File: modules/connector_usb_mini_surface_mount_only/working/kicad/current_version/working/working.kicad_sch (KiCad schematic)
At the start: 1 part, among them J1 scumnsmo

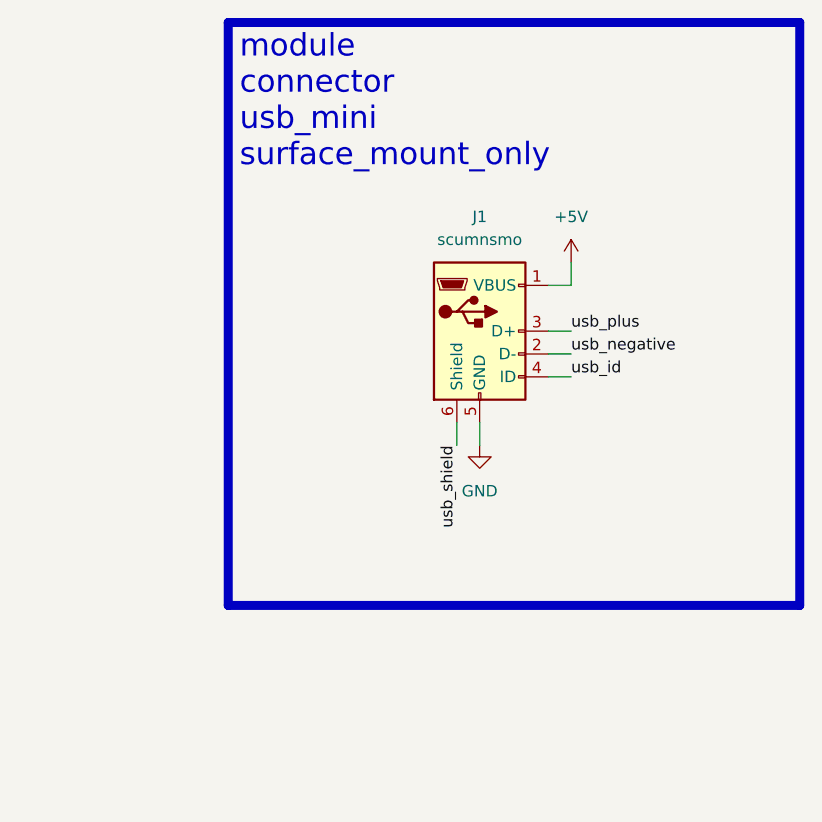
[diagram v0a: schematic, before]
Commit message: a few module workings
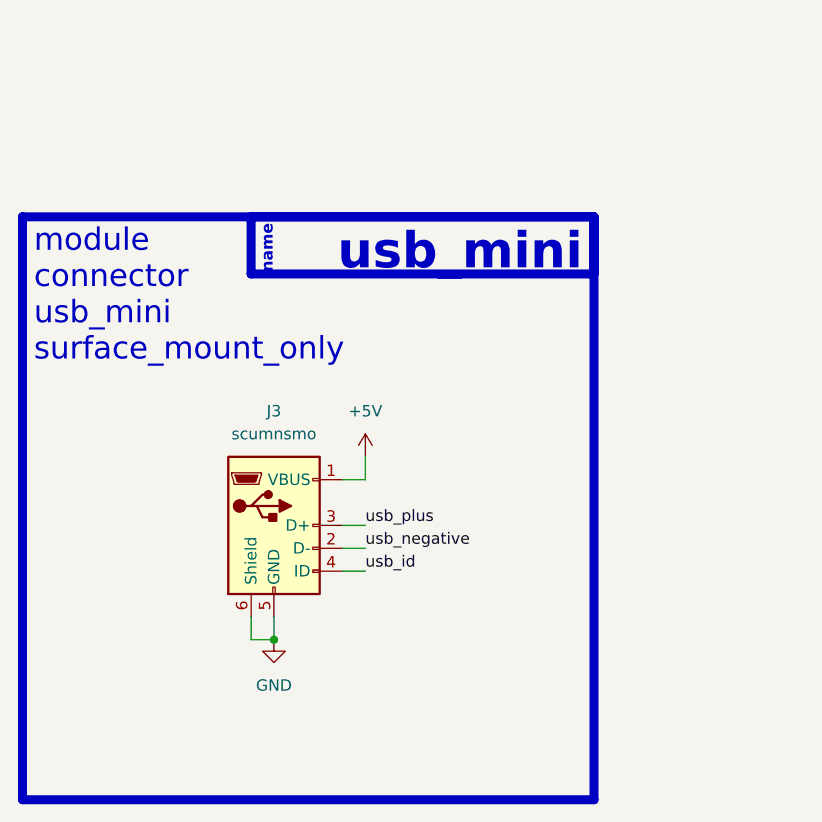
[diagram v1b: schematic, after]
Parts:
- removed J1: scumnsmo, scumnsmo_electronic_socket_usb_mini_surface_mount_only, symbol oomlout_oomp_part_symbols:scumnsmo_electronic_socket_usb_mini_surface_mount_only
- added J3: scumnsmo, oomlout_oomp_part_kicad_footprints:scumnsmo_electronic_socket_usb_mini_surface_mount_only, symbol oomlout_oomp_part_symbols:scumnsmo_electronic_socket_usb_mini_surface_mount_only
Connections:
- net +5V: now also J3.1 (VBUS)
- net GND: now also J3.5 (GND), J3.6 (Shield)
- net usb_id: now also J3.4 (ID)
- net usb_negative: now also J3.2 (D-)
- net usb_plus: now also J3.3 (D+)
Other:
- note added: "name"
- note added: "usb_mini"
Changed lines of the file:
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@@
 (kicad_sch (version 20230121) (generator eeschema)
   (paper "A4")
-  (wire (pts (xy 175.26 69.85) (xy 172.72 69.85))
+  (junction (at 142.24 109.22) (diameter 0) (color 0 0 0 0)
+  )
+  (wire (pts (xy 149.86 96.52) (xy 152.4 96.52))
     (stroke (width 0) (type default))
   )
-  (wire (pts (xy 165.1 85.09) (xy 165.1 87.63))
+  (wire (pts (xy 142.24 106.68) (xy 142.24 109.22))
     (stroke (width 0) (type default))
   )
-  (wire (pts (xy 162.56 85.09) (xy 162.56 87.63))
+  (wire (pts (xy 152.4 91.44) (xy 149.86 91.44))
     (stroke (width 0) (type default))
   )
-  (wire (pts (xy 172.72 74.93) (xy 175.26 74.93))
+  (wire (pts (xy 139.7 106.68) (xy 139.7 109.22))
     (stroke (width 0) (type default))
   )
-  (wire (pts (xy 172.72 80.01) (xy 175.26 80.01))
+  (wire (pts (xy 149.86 99.06) (xy 152.4 99.06))
     (stroke (width 0) (type default))
   )
-  (wire (pts (xy 175.26 67.31) (xy 175.26 69.85))
+  (wire (pts (xy 139.7 109.22) (xy 142.24 109.22))
     (stroke (width 0) (type default))
   )
-  (wire (pts (xy 172.72 77.47) (xy 175.26 77.47))
+  (wire (pts (xy 149.86 101.6) (xy 152.4 101.6))
     (stroke (width 0) (type default))
   )
-  (rectangle (start 137.16 40.64) (end 200.66 105.41)
+  (wire (pts (xy 152.4 88.9) (xy 152.4 91.44))
+    (stroke (width 0) (type default))
+  )
+  (rectangle (start 139.7 62.23) (end 177.8 68.58)
+    (stroke (width 1) (type default))
+    (fill (type color) (color 0 0 0 0))
+  )
+  (rectangle (start 114.3 62.23) (end 177.8 127)
     (stroke (width 1) (type default))
     (fill (type none))
   )
-  (rectangle (start 199.39 97.79) (end 199.39 97.79)
-    (stroke (width 0) (type default))
-    (fill (type none))
-  )
-  (text "module\nconnector\nusb_mini\nsurface_mount_only\n\n" (at 138.43 60.96 0)
+  (text "module\nconnector\nusb_mini\nsurface_mount_only\n\n" (at 115.57 82.55 0)
     (effects (font (size 2.5 2.5)) (justify left bottom))
   )
-  (label "usb_id" (at 175.26 80.01 0) (fields_autoplaced)
+  (text "name" (at 142.24 68.58 90)
+    (effects (font (size 1.27 1.27) (thickness 0.254) bold (color 255 255 255 1)) (justify left bottom))
+  )
+  (text "usb_mini\n" (at 176.53 68.58 0)
+    (effects (font (size 4 4) (thickness 0.8) bold (color 255 255 255 1)) (justify right bottom))
+  )
+  (label "usb_negative" (at 152.4 99.06 0) (fields_autoplaced)
     (effects (font (size 1.27 1.27)) (justify left bottom))
   )
-  (label "usb_plus" (at 175.26 74.93 0) (fields_autoplaced)
+  (label "usb_id" (at 152.4 101.6 0) (fields_autoplaced)
     (effects (font (size 1.27 1.27)) (justify left bottom))
   )
-  (label "usb_negative" (at 175.26 77.47 0) (fields_autoplaced)
+  (label "usb_plus" (at 152.4 96.52 0) (fields_autoplaced)
     (effects (font (size 1.27 1.27)) (justify left bottom))
   )
-  (label "usb_shield" (at 162.56 87.63 270) (fields_autoplaced)
-    (effects (font (size 1.27 1.27)) (justify right bottom))
-  )
-  (symbol (lib_id "oomlout_oomp_part_symbols:scumnsmo_electronic_socket_usb_mini_surface_mount_only") (at 165.1 74.93 0) (unit 1)
+  (symbol (lib_id "power:+5V") (at 152.4 88.9 0) (unit 1)
     (in_bom yes) (on_board yes) (dnp no) (fields_autoplaced)
-    (property "Reference" "J1" (at 165.1 62.23 0)
+    (property "Reference" "#PWR013" (at 152.4 92.71 0)
+      (effects (font (size 1.27 1.27)) hide)
+    )
+    (property "Value" "+5V" (at 152.4 83.82 0)
       (effects (font (size 1.27 1.27)))
     )
-    (property "Value" "scumnsmo" (at 165.1 64.77 0)
+    (property "Footprint" "" (at 152.4 88.9 0)
+      (effects (font (size 1.27 1.27)) hide)
+    )
+    (property "Datasheet" "" (at 152.4 88.9 0)
+      (effects (font (size 1.27 1.27)) hide)
+    )
+    (pin "1")
+    (instances
+      (project "working"
+        (path "/5407c114-4107-4d84-8382-1717fb9d687c"
+          (reference "#PWR013") (unit 1)
+        )
+      )
+      (project "working"
+        (path "/d7ac9d55-1973-40f4-b2a5-38a433b49fa0"
+          (reference "#PWR02") (unit 1)
+        )
+      )
+    )
+  )
+  (symbol (lib_id "oomlout_oomp_part_symbols:scumnsmo_electronic_socket_usb_mini_surface_mount_only") (at 142.24 96.52 0) (unit 1)
+    (in_bom yes) (on_board yes) (dnp no) (fields_autoplaced)
+    (property "Reference" "J3" (at 142.24 83.82 0)
       (effects (font (size 1.27 1.27)))
     )
-    (property "Footprint" "scumnsmo_electronic_socket_usb_mini_surface_mount_only" (at 168.91 76.2 0)
+    (property "Value" "scumnsmo" (at 142.24 86.36 0)
+      (effects (font (size 1.27 1.27)))
+    )
+    (property "Footprint" "oomlout_oomp_part_kicad_footprints:scumnsmo_electronic_socket_usb_mini_surface_mount_only" (at 146.05 97.79 0)
       (effects (font (size 1.27 1.27)) hide)
     )
-    (property "Datasheet" "https://github.com/oomlout/oomlout_oomp_v3/parts/electronic_socket_usb_mini_surface_mount_only/datasheet.pdf" (at 168.91 76.2 0)
+    (property "Datasheet" "https://github.com/oomlout/oomlout_oomp_v3/parts/electronic_socket_usb_mini_surface_mount_only/datasheet.pdf" (at 146.05 97.79 0)
       (effects (font (size 1.27 1.27)) hide)
     )
@@
     (instances
       (project "working"
+        (path "/5407c114-4107-4d84-8382-1717fb9d687c"
+          (reference "J3") (unit 1)
+        )
+      )
+      (project "working"
         (path "/d7ac9d55-1973-40f4-b2a5-38a433b49fa0"
           (reference "J1") (unit 1)
@@
     )
   )
-  (symbol (lib_id "power:+5V") (at 175.26 67.31 0) (unit 1)
+  (symbol (lib_id "power:GND") (at 142.24 109.22 0) (unit 1)
     (in_bom yes) (on_board yes) (dnp no) (fields_autoplaced)
-    (property "Reference" "#PWR04" (at 175.26 71.12 0)
+    (property "Reference" "#PWR012" (at 142.24 115.57 0)
       (effects (font (size 1.27 1.27)) hide)
     )
-    (property "Value" "+5V" (at 175.26 62.23 0)
+    (property "Value" "GND" (at 142.24 114.3 0)
       (effects (font (size 1.27 1.27)))
     )
-    (property "Footprint" "" (at 175.26 67.31 0)
+    (property "Footprint" "" (at 142.24 109.22 0)
       (effects (font (size 1.27 1.27)) hide)
     )
-    (property "Datasheet" "" (at 175.26 67.31 0)
+    (property "Datasheet" "" (at 142.24 109.22 0)
       (effects (font (size 1.27 1.27)) hide)
     )
@@
     (instances
       (project "working"
-        (path "/d7ac9d55-1973-40f4-b2a5-38a433b49fa0"
-          (reference "#PWR04") (unit 1)
+        (path "/5407c114-4107-4d84-8382-1717fb9d687c"
+          (reference "#PWR012") (unit 1)
         )
       )
-    )
-  )
-  (symbol (lib_id "power:GND") (at 165.1 87.63 0) (unit 1)
-    (in_bom yes) (on_board yes) (dnp no) (fields_autoplaced)
-    (property "Reference" "#PWR03" (at 165.1 93.98 0)
-      (effects (font (size 1.27 1.27)) hide)
-    )
-    (property "Value" "GND" (at 165.1 92.71 0)
-      (effects (font (size 1.27 1.27)))
-    )
-    (property "Footprint" "" (at 165.1 87.63 0)
-      (effects (font (size 1.27 1.27)) hide)
-    )
-    (property "Datasheet" "" (at 165.1 87.63 0)
-      (effects (font (size 1.27 1.27)) hide)
-    )
-    (pin "1")
-    (instances
       (project "working"
         (path "/d7ac9d55-1973-40f4-b2a5-38a433b49fa0"
-          (reference "#PWR03") (unit 1)
+          (reference "#PWR01") (unit 1)
         )
       )

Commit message: works.
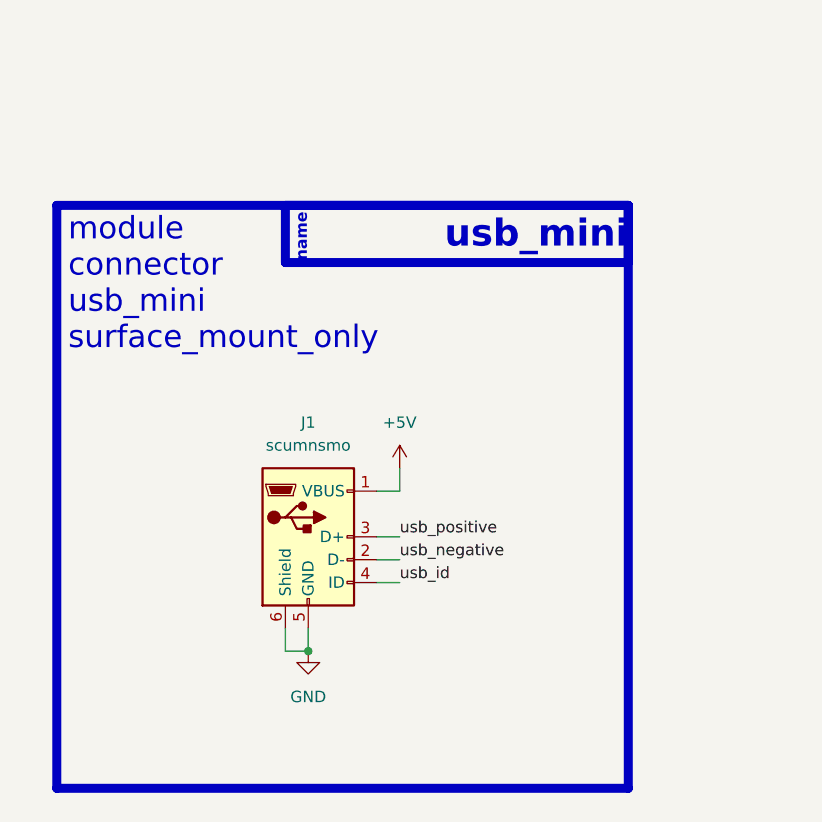
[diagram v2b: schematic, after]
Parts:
- removed J3: scumnsmo, oomlout_oomp_part_kicad_footprints:scumnsmo_electronic_socket_usb_mini_surface_mount_only, symbol oomlout_oomp_part_symbols:scumnsmo_electronic_socket_usb_mini_surface_mount_only
- added J1: scumnsmo, oomlout_oomp_part_footprints:scumnsmo_electronic_socket_usb_mini_surface_mount_only, symbol oomlout_oomp_part_symbols:scumnsmo_electronic_socket_usb_mini_surface_mount_only
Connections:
- net +5V: now also J1.1 (VBUS)
- net GND: now also J1.5 (GND), J1.6 (Shield)
- net usb_id: now also J1.4 (ID)
- net usb_negative: now also J1.2 (D-)
- new net usb_positive: J1.3 (D+)
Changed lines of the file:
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@@
 (kicad_sch (version 20230121) (generator eeschema)
   (paper "A4")
-  (junction (at 142.24 109.22) (diameter 0) (color 0 0 0 0)
+  (junction (at 146.05 110.49) (diameter 0) (color 0 0 0 0)
   )
-  (wire (pts (xy 149.86 96.52) (xy 152.4 96.52))
+  (wire (pts (xy 153.67 102.87) (xy 156.21 102.87))
     (stroke (width 0) (type default))
   )
-  (wire (pts (xy 142.24 106.68) (xy 142.24 109.22))
+  (wire (pts (xy 146.05 107.95) (xy 146.05 110.49))
     (stroke (width 0) (type default))
   )
-  (wire (pts (xy 152.4 91.44) (xy 149.86 91.44))
+  (wire (pts (xy 156.21 90.17) (xy 156.21 92.71))
     (stroke (width 0) (type default))
   )
-  (wire (pts (xy 139.7 106.68) (xy 139.7 109.22))
+  (wire (pts (xy 153.67 97.79) (xy 156.21 97.79))
     (stroke (width 0) (type default))
   )
-  (wire (pts (xy 149.86 99.06) (xy 152.4 99.06))
+  (wire (pts (xy 143.51 110.49) (xy 146.05 110.49))
     (stroke (width 0) (type default))
   )
-  (wire (pts (xy 139.7 109.22) (xy 142.24 109.22))
+  (wire (pts (xy 153.67 92.71) (xy 156.21 92.71))
     (stroke (width 0) (type default))
   )
-  (wire (pts (xy 149.86 101.6) (xy 152.4 101.6))
+  (wire (pts (xy 143.51 107.95) (xy 143.51 110.49))
     (stroke (width 0) (type default))
   )
-  (wire (pts (xy 152.4 88.9) (xy 152.4 91.44))
+  (wire (pts (xy 153.67 100.33) (xy 156.21 100.33))
     (stroke (width 0) (type default))
   )
-  (rectangle (start 139.7 62.23) (end 177.8 68.58)
+  (rectangle (start 118.11 60.96) (end 181.61 125.73)
+    (stroke (width 1) (type default))
+    (fill (type none))
+  )
+  (rectangle (start 143.51 60.96) (end 181.61 67.31)
     (stroke (width 1) (type default))
     (fill (type color) (color 0 0 0 0))
   )
-  (rectangle (start 114.3 62.23) (end 177.8 127)
-    (stroke (width 1) (type default))
-    (fill (type none))
+  (text "usb_mini" (at 181.61 66.04 0)
+    (effects (font (size 3 3) (thickness 0.8) bold (color 255 255 255 1)) (justify right bottom))
   )
-  (text "module\nconnector\nusb_mini\nsurface_mount_only\n\n" (at 115.57 82.55 0)
+  (text "name" (at 146.05 67.31 90)
+    (effects (font (size 1.27 1.27) (thickness 0.254) bold (color 255 255 255 1)) (justify left bottom))
+  )
+  (text "module\nconnector\nusb_mini\nsurface_mount_only\n\n" (at 119.38 81.28 0)
     (effects (font (size 2.5 2.5)) (justify left bottom))
   )
-  (text "name" (at 142.24 68.58 90)
-    (effects (font (size 1.27 1.27) (thickness 0.254) bold (color 255 255 255 1)) (justify left bottom))
-  )
-  (text "usb_mini\n" (at 176.53 68.58 0)
-    (effects (font (size 4 4) (thickness 0.8) bold (color 255 255 255 1)) (justify right bottom))
-  )
-  (label "usb_negative" (at 152.4 99.06 0) (fields_autoplaced)
+  (label "usb_id" (at 156.21 102.87 0) (fields_autoplaced)
     (effects (font (size 1.27 1.27)) (justify left bottom))
   )
-  (label "usb_id" (at 152.4 101.6 0) (fields_autoplaced)
+  (label "usb_positive" (at 156.21 97.79 0) (fields_autoplaced)
     (effects (font (size 1.27 1.27)) (justify left bottom))
   )
-  (label "usb_plus" (at 152.4 96.52 0) (fields_autoplaced)
+  (label "usb_negative" (at 156.21 100.33 0) (fields_autoplaced)
     (effects (font (size 1.27 1.27)) (justify left bottom))
   )
-  (symbol (lib_id "power:+5V") (at 152.4 88.9 0) (unit 1)
+  (symbol (lib_id "power:GND") (at 146.05 110.49 0) (unit 1)
     (in_bom yes) (on_board yes) (dnp no) (fields_autoplaced)
-    (property "Reference" "#PWR013" (at 152.4 92.71 0)
+    (property "Reference" "#PWR012" (at 146.05 116.84 0)
       (effects (font (size 1.27 1.27)) hide)
     )
-    (property "Value" "+5V" (at 152.4 83.82 0)
+    (property "Value" "GND" (at 146.05 115.57 0)
       (effects (font (size 1.27 1.27)))
     )
-    (property "Footprint" "" (at 152.4 88.9 0)
+    (property "Footprint" "" (at 146.05 110.49 0)
       (effects (font (size 1.27 1.27)) hide)
     )
-    (property "Datasheet" "" (at 152.4 88.9 0)
+    (property "Datasheet" "" (at 146.05 110.49 0)
+      (effects (font (size 1.27 1.27)) hide)
+    )
+    (pin "1")
+    (instances
+      (project "working"
+        (path "/5407c114-4107-4d84-8382-1717fb9d687c"
+          (reference "#PWR012") (unit 1)
+        )
+      )
+      (project "working"
+        (path "/d7ac9d55-1973-40f4-b2a5-38a433b49fa0"
+          (reference "#PWR01") (unit 1)
+        )
+      )
+    )
+  )
+  (symbol (lib_id "power:+5V") (at 156.21 90.17 0) (unit 1)
+    (in_bom yes) (on_board yes) (dnp no) (fields_autoplaced)
+    (property "Reference" "#PWR013" (at 156.21 93.98 0)
+      (effects (font (size 1.27 1.27)) hide)
+    )
+    (property "Value" "+5V" (at 156.21 85.09 0)
+      (effects (font (size 1.27 1.27)))
+    )
+    (property "Footprint" "" (at 156.21 90.17 0)
+      (effects (font (size 1.27 1.27)) hide)
+    )
+    (property "Datasheet" "" (at 156.21 90.17 0)
       (effects (font (size 1.27 1.27)) hide)
     )
@@
     )
   )
-  (symbol (lib_id "oomlout_oomp_part_symbols:scumnsmo_electronic_socket_usb_mini_surface_mount_only") (at 142.24 96.52 0) (unit 1)
+  (symbol (lib_id "oomlout_oomp_part_symbols:scumnsmo_electronic_socket_usb_mini_surface_mount_only") (at 146.05 97.79 0) (unit 1)
     (in_bom yes) (on_board yes) (dnp no) (fields_autoplaced)
-    (property "Reference" "J3" (at 142.24 83.82 0)
+    (property "Reference" "J1" (at 146.05 85.09 0)
       (effects (font (size 1.27 1.27)))
     )
-    (property "Value" "scumnsmo" (at 142.24 86.36 0)
+    (property "Value" "scumnsmo" (at 146.05 87.63 0)
       (effects (font (size 1.27 1.27)))
     )
-    (property "Footprint" "oomlout_oomp_part_kicad_footprints:scumnsmo_electronic_socket_usb_mini_surface_mount_only" (at 146.05 97.79 0)
+    (property "Footprint" "oomlout_oomp_part_footprints:scumnsmo_electronic_socket_usb_mini_surface_mount_only" (at 149.86 99.06 0)
       (effects (font (size 1.27 1.27)) hide)
     )
-    (property "Datasheet" "https://github.com/oomlout/oomlout_oomp_v3/parts/electronic_socket_usb_mini_surface_mount_only/datasheet.pdf" (at 146.05 97.79 0)
+    (property "Datasheet" "https://github.com/oomlout/oomlout_oomp_v3/parts/electronic_socket_usb_mini_surface_mount_only/datasheet.pdf" (at 149.86 99.06 0)
       (effects (font (size 1.27 1.27)) hide)
     )
@@
     (instances
       (project "working"
-        (path "/5407c114-4107-4d84-8382-1717fb9d687c"
-          (reference "J3") (unit 1)
-        )
-      )
-      (project "working"
         (path "/d7ac9d55-1973-40f4-b2a5-38a433b49fa0"
           (reference "J1") (unit 1)
         )
       )
-    )
-  )
-  (symbol (lib_id "power:GND") (at 142.24 109.22 0) (unit 1)
-    (in_bom yes) (on_board yes) (dnp no) (fields_autoplaced)
-    (property "Reference" "#PWR012" (at 142.24 115.57 0)
-      (effects (font (size 1.27 1.27)) hide)
-    )
-    (property "Value" "GND" (at 142.24 114.3 0)
-      (effects (font (size 1.27 1.27)))
-    )
-    (property "Footprint" "" (at 142.24 109.22 0)
-      (effects (font (size 1.27 1.27)) hide)
-    )
-    (property "Datasheet" "" (at 142.24 109.22 0)
-      (effects (font (size 1.27 1.27)) hide)
-    )
-    (pin "1")
-    (instances
-      (project "working"
-        (path "/5407c114-4107-4d84-8382-1717fb9d687c"
-          (reference "#PWR012") (unit 1)
-        )
-      )
-      (project "working"
-        (path "/d7ac9d55-1973-40f4-b2a5-38a433b49fa0"
-          (reference "#PWR01") (unit 1)
-        )
-      )
